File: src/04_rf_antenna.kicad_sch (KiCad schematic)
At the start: 0 parts

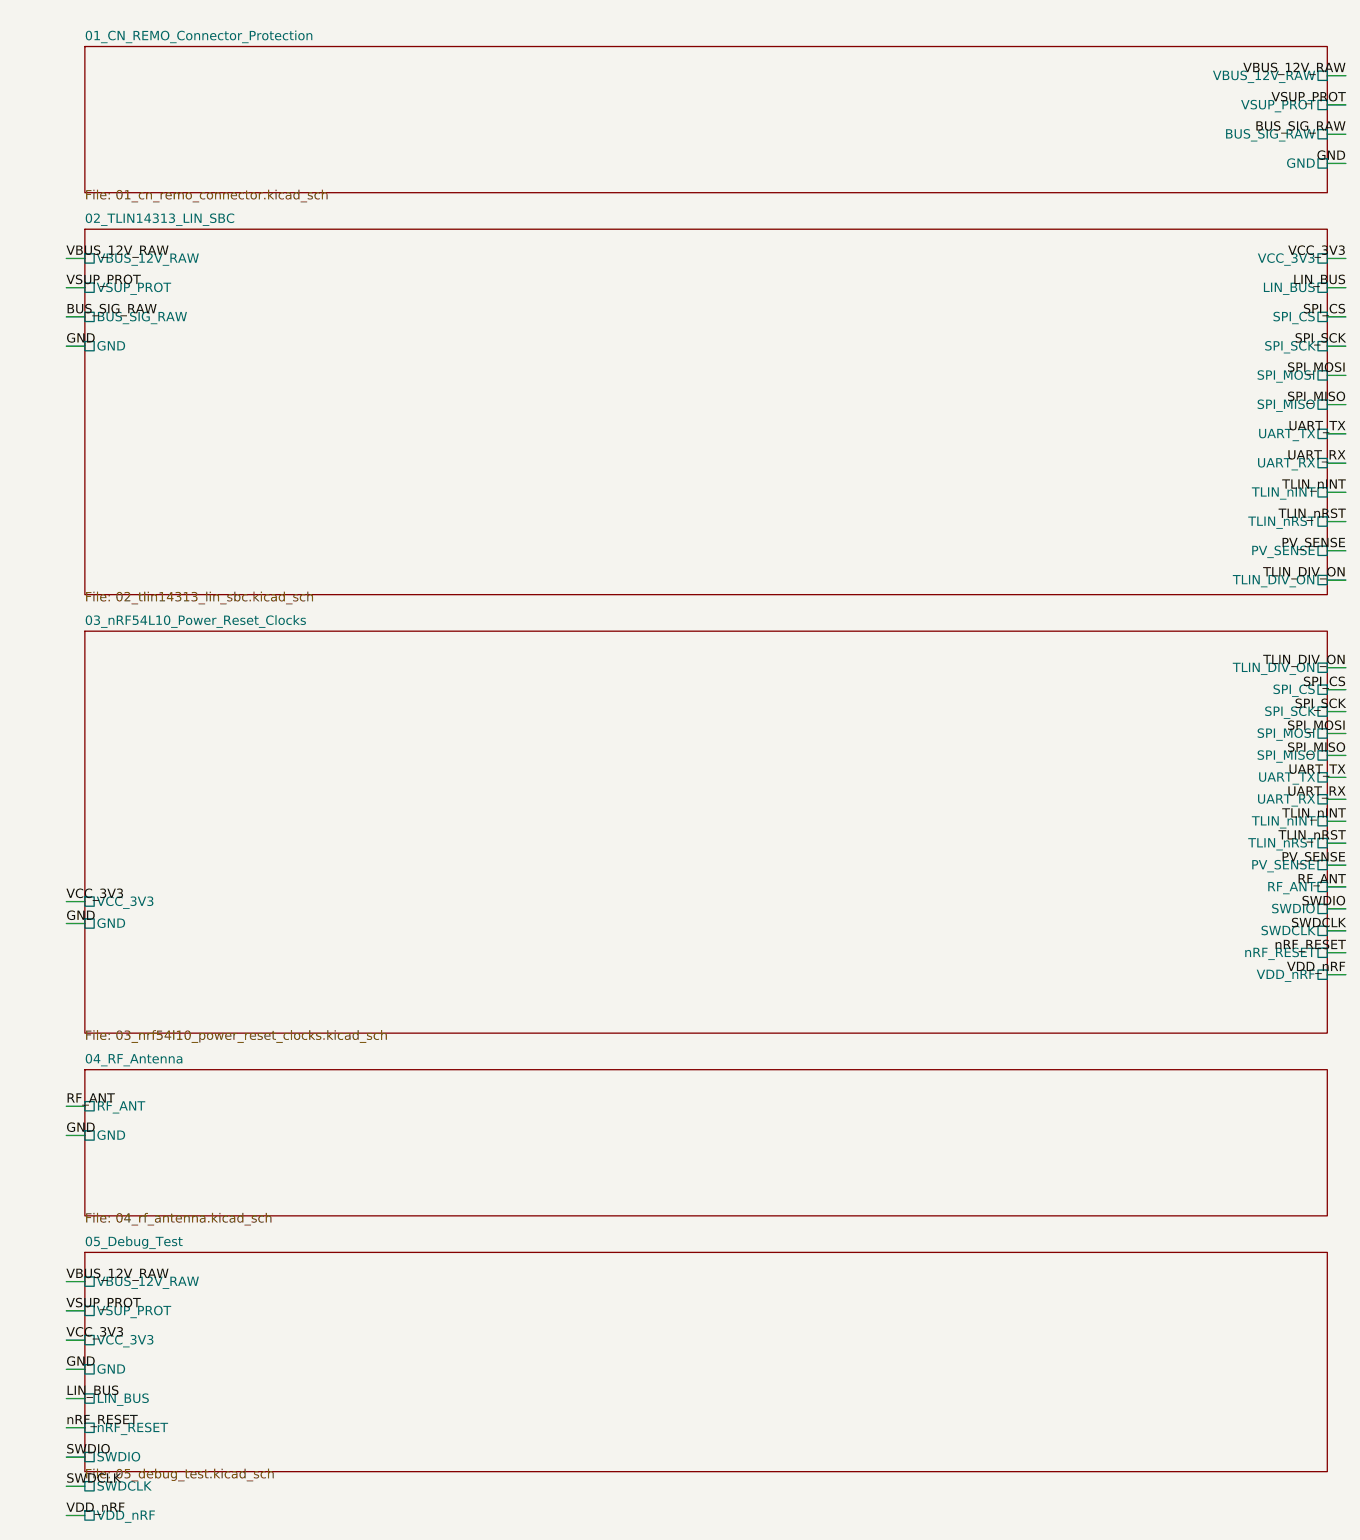
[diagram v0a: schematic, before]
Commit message: stage
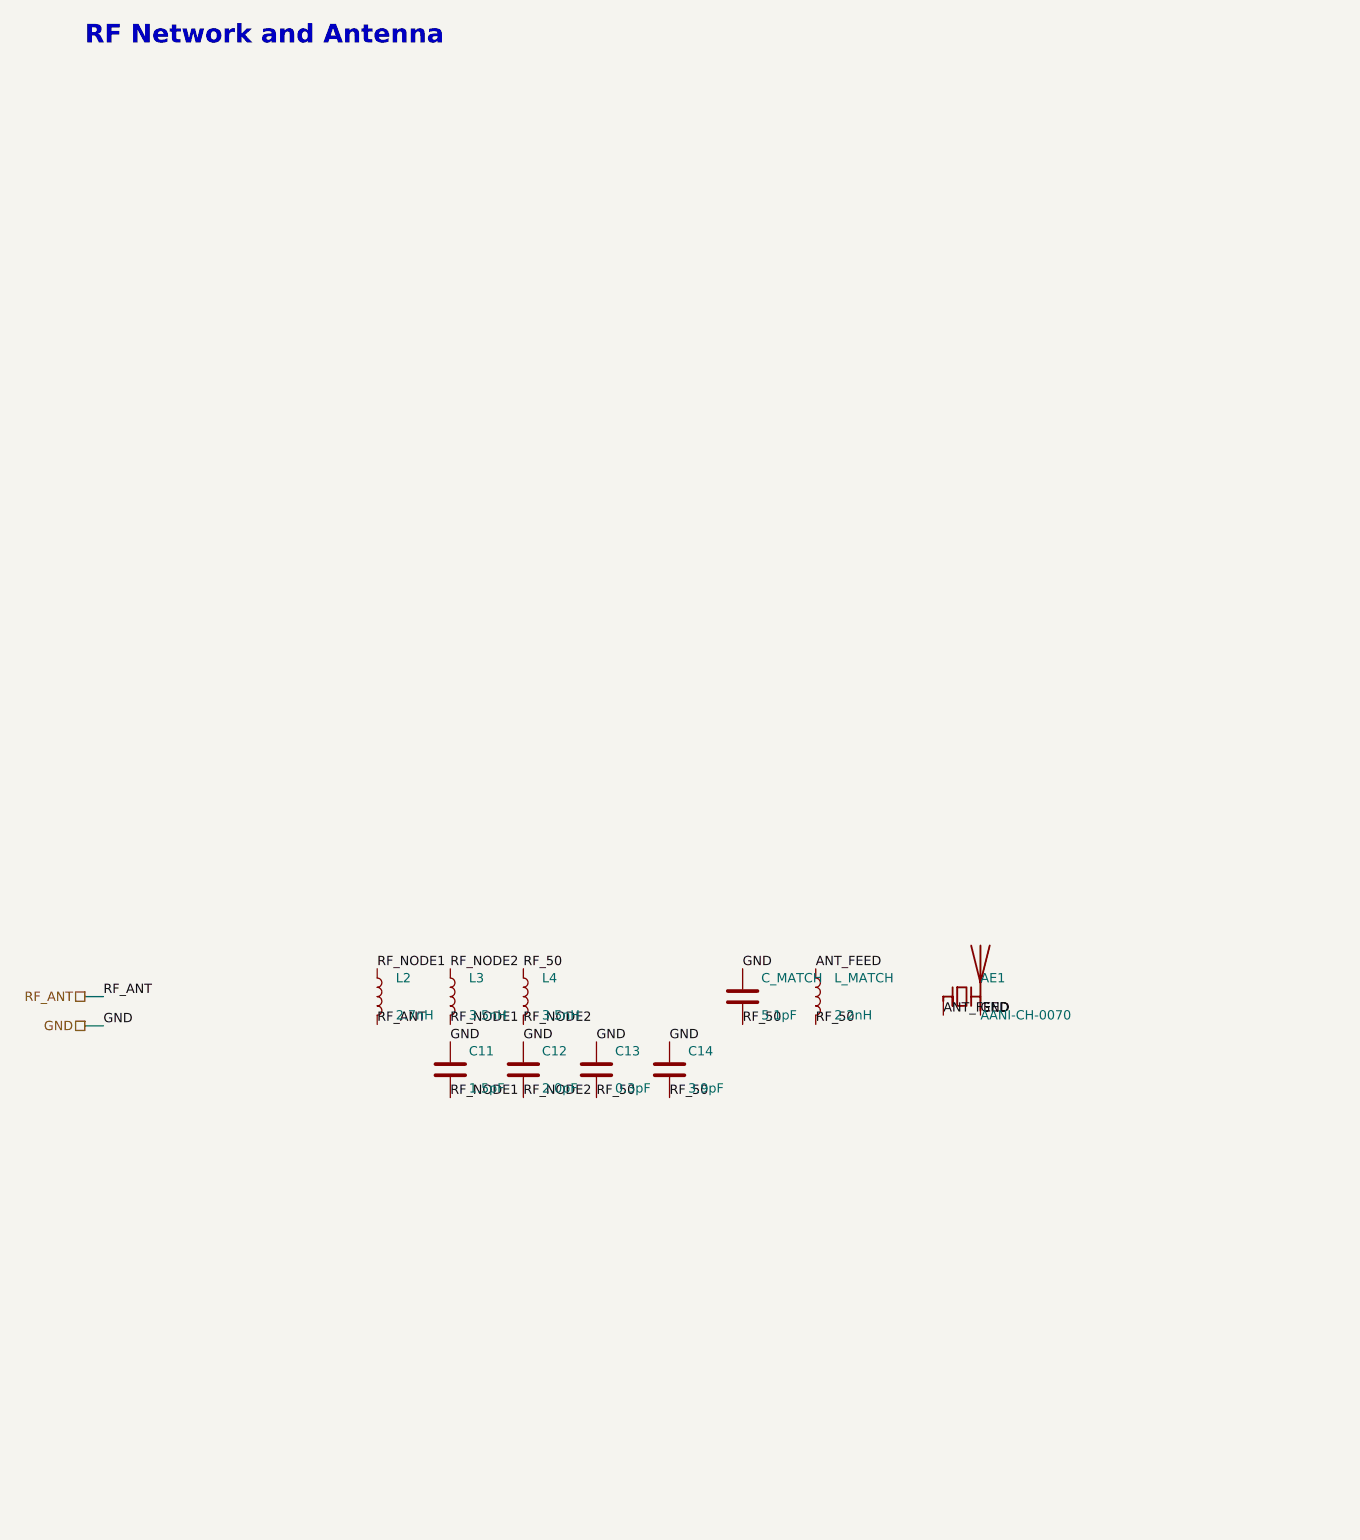
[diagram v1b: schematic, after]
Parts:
- added AE1: AANI-CH-0070, symbol Device:Antenna_Chip
- added C11: 1.5pF, symbol Device:C
- added C12: 2.0pF, symbol Device:C
- added C13: 0.3pF, symbol Device:C
- added C14: 3.9pF, symbol Device:C
- added C_MATCH: 5.1pF, symbol Device:C
- added L2: 2.7nH, symbol Device:L
- added L3, L4: 3.5nH, symbol Device:L
- added L_MATCH: 2.2nH, symbol Device:L
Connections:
- net GND: now also AE1.2 (PCB_Trace), C11.1, C12.1, C13.1, C14.1, C_MATCH.1
- net RF_ANT: now also L2.2
- new net ANT_FEED: AE1.1 (FEED), L_MATCH.1
- new net RF_50: C13.2, C14.2, C_MATCH.2, L4.1, L_MATCH.2
- new net RF_NODE1: C11.2, L2.1, L3.2
- new net RF_NODE2: C12.2, L3.1, L4.2
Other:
- removed sheet 01_CN_REMO_Connector_Protection
- removed sheet 02_TLIN14313_LIN_SBC
- removed sheet 03_nRF54L10_Power_Reset_Clocks
- removed sheet 04_RF_Antenna
- removed sheet 05_Debug_Test
- note added: "RF Network and Antenna"
